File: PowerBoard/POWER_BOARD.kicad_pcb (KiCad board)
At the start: 4 copper layers, 152.1 x 80.1 mm, 158 parts, among them J1 B3B-XH-A_LF__SN_, J2 USB4145-03-0170-C_REVA2, J3 Molex Microfit 3.0, J5 Conn_02x10_Counter_Clockwise, J6 Molex Microfit 3.0, Q1 BSS138, Q2 FDD86250-F085, Q3 FGH50T65SQD-F155, Q4 BSS138, Q5 TN2130K1-G, Q6 STD11N60DM2, Q7 FGH50T65SQD-F155, T1 DA2034, U1 RPI2040, U10 PTS647SM38SMTR2LFS, U2 MCP14A0454-E/SN, U3 NCV1117DT33T5G, U4 LT3750, U5 W25Q16JVSNIQ, U6 LTC4151IMS_PBF, U7 MCP2515-xST, U8 MCP2551-I-SN, U9 PTS647SM38SMTR2LFS, Y1 ABM3-12.000MHZ-D2Y-T, Y2 ABM3-8.000MHZ-D2Y-T

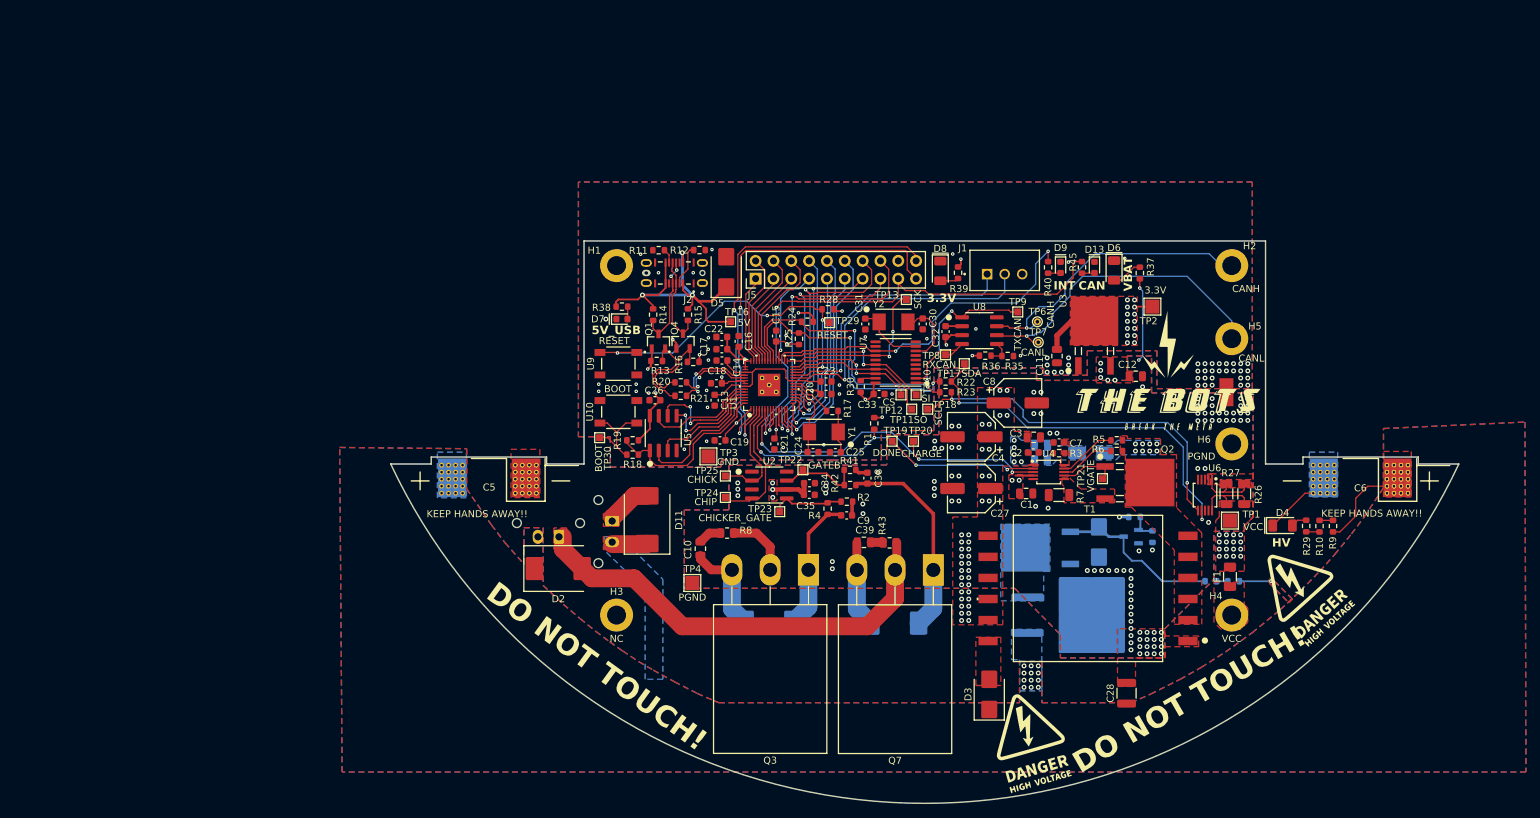
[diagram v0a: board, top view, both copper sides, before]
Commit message: added pdfs
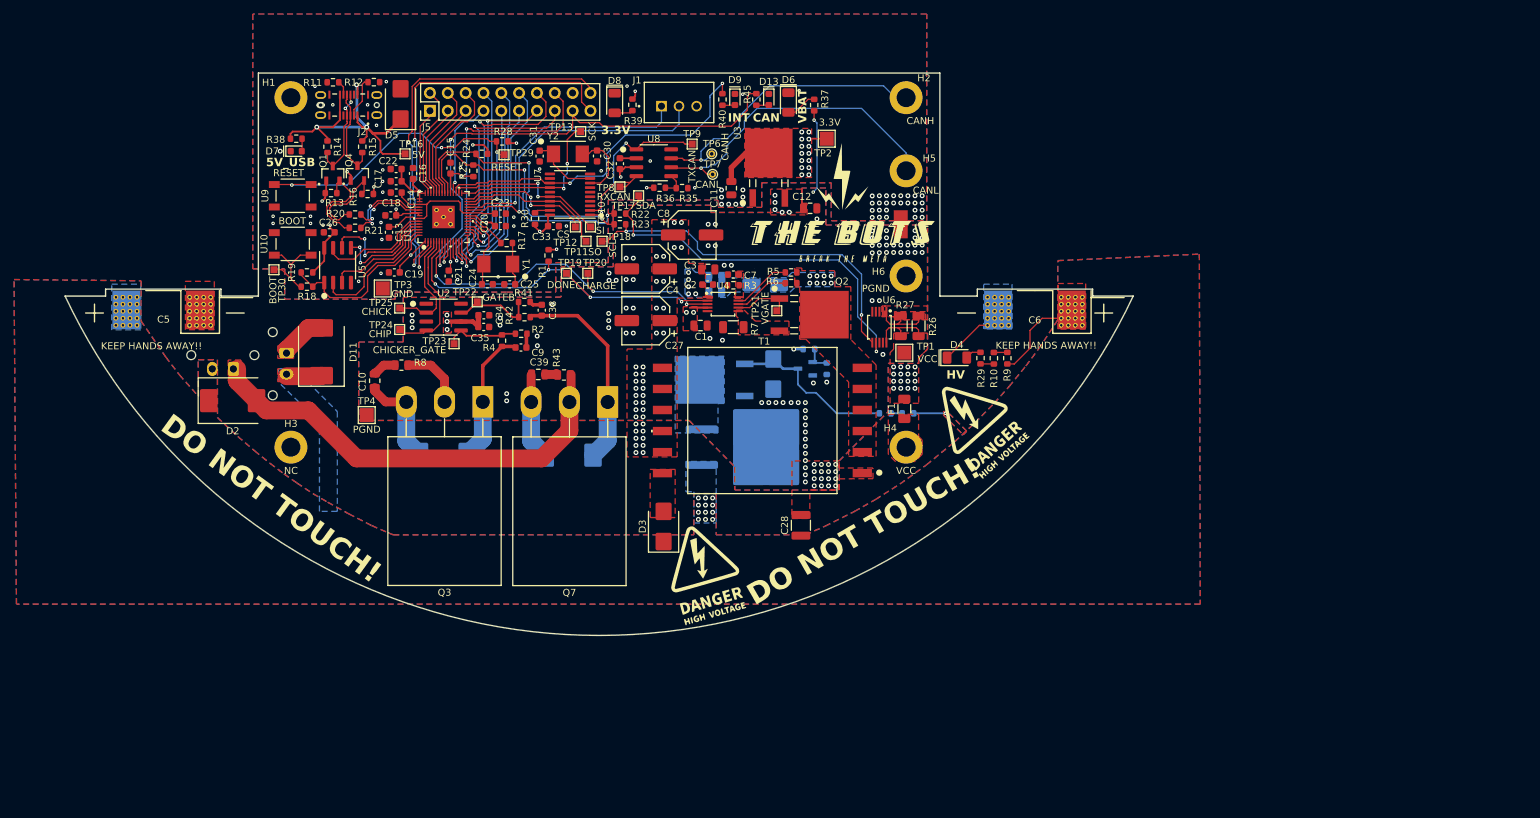
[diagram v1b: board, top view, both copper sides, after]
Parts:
- moved C2 52.2 mm to (119.7, 62.1)
- moved C3 52.2 mm to (119.7, 60.0)
- moved TP22 52.2 mm to (86.8, 64.6)
- moved R1 52.2 mm to (97.0, 58.0)
- moved R14 52.2 mm to (65.5, 42.5)
- moved R15 52.2 mm to (70.5, 42.5)
- moved R25 52.2 mm to (86.3, 45.9)
- moved TP17 52.2 mm to (109.8, 49.5)
- moved TP2 52.2 mm to (136.6, 41.4)
- moved TP9 52.2 mm to (117.4, 42.1)
- moved C13 52.2 mm to (74.3, 54.7)
- moved C15 52.2 mm to (83.0, 45.6)
- moved C19 52.2 mm to (75.0, 60.4)
- moved C20 52.2 mm to (90.1, 53.8)
- moved C23 52.2 mm to (90.1, 52.0)
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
